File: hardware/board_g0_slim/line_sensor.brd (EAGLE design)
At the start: 100 x 31.3 mm, 62 parts, among them J1 XF2L-0535-1, Q1 BSS123

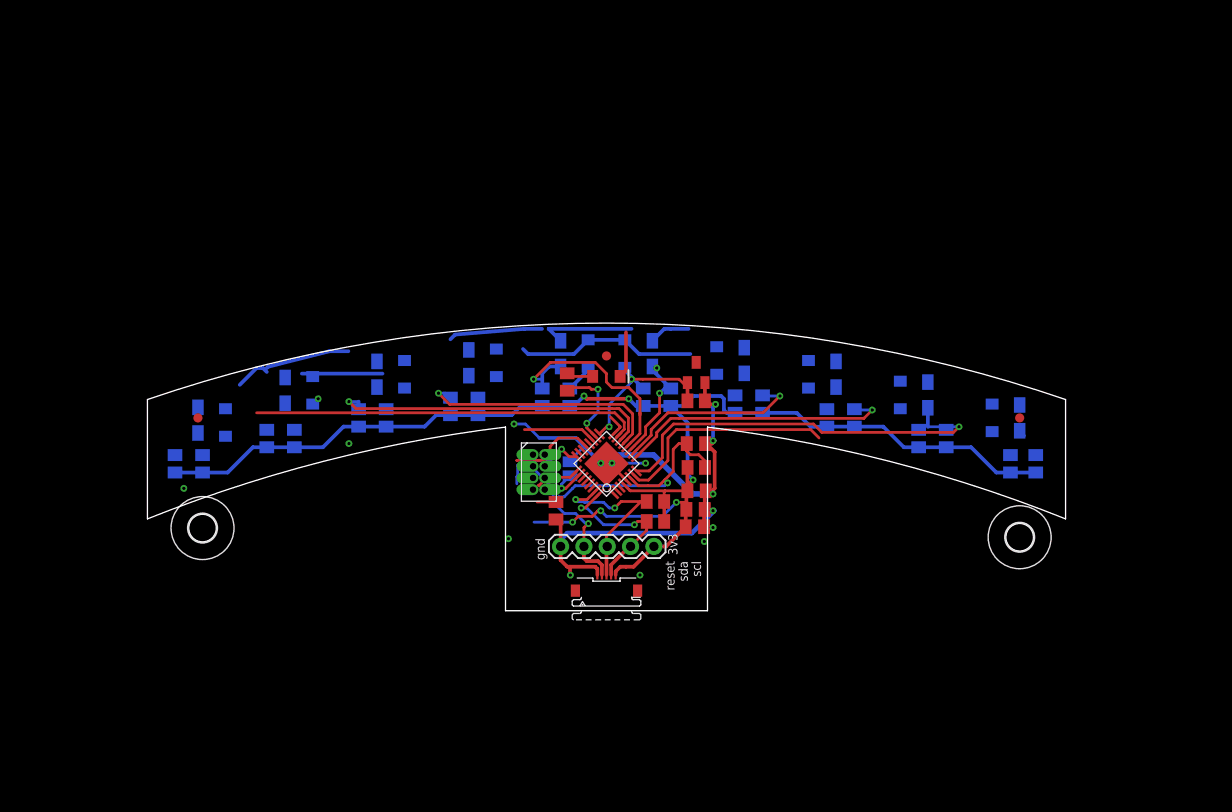
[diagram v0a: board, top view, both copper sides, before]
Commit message: demo codes, cleaned up
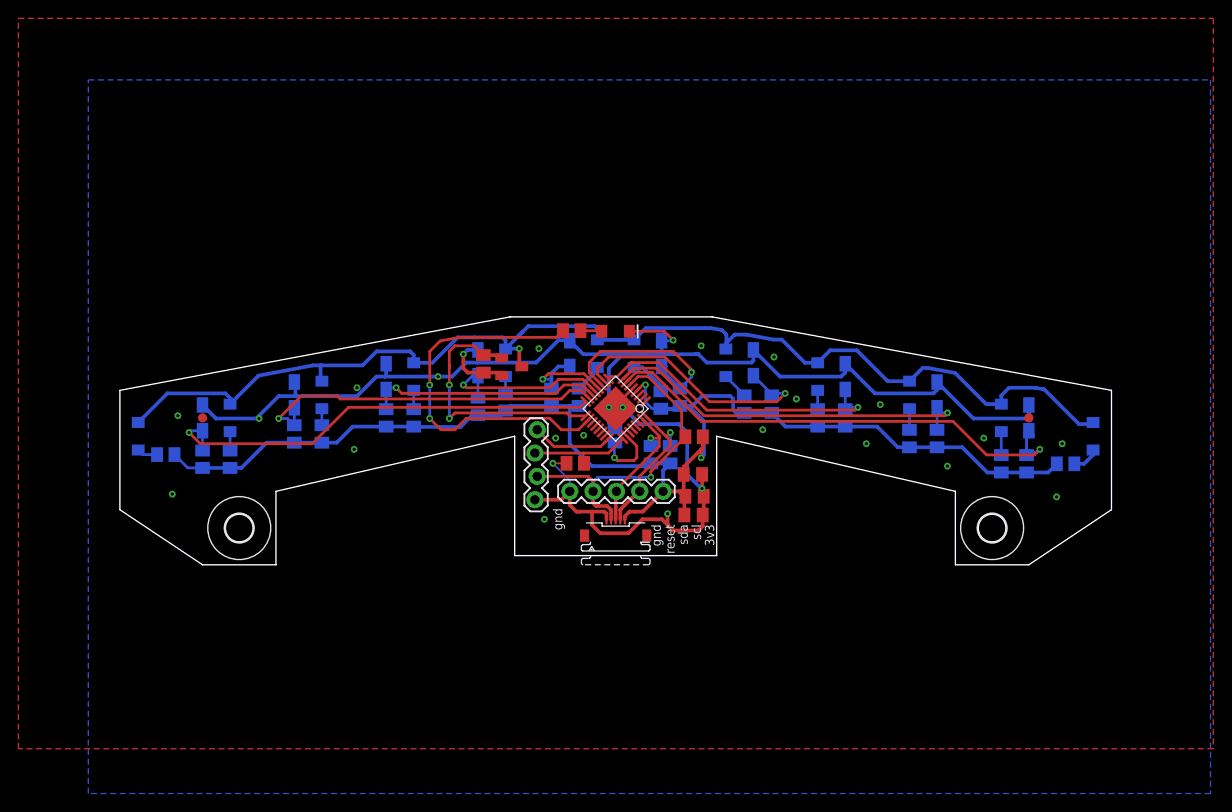
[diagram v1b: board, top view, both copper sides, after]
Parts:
- removed C4: 10n, rcl:C0805K
- removed U$11: FIDUCIAL, borkedlabs-misc:FIDUCIAL_1MM
- removed U$15: DEBUG_CON, my_library:HEADER_4X2_1.27
- added D12, D13: WHITE, SparkFun-LED:LED-1206
- added J3: (no value), SparkFun-Connectors:1X04_LOCK
- added R27, R28: 330, rcl:M0805
- moved R21 23.5 mm to (40.6, 45.9), turned to 90 degrees
- moved Q1 20.1 mm to (43.7, 45.6), turned to 270 degrees
- moved R23 7.44 mm to (60.9, 36.0), flipped to the bottom, turned to 270 degrees
- moved J1 6.08 mm to (55.0, 27.0)
- moved J2 6.08 mm to (50.0, 32.0)
- moved U$14 6.08 mm to (55.0, 41.0), turned to 225 degrees
- moved SJ1 6.06 mm to (54.9, 38.0)
- moved C2 5.70 mm to (63.4, 33.8)
- moved R26 5.61 mm to (50.2, 49.5), turned to 180 degrees
- moved R25 5.57 mm to (50.6, 35.1), turned to 0 degrees
- moved R22 5.12 mm to (58.8, 36.0), flipped to the bottom, turned to 270 degrees
- moved D11 5.02 mm to (55.0, 49.4)
- moved H8 4.00 mm to (14.0, 28.0)
- moved R24 3.34 mm to (63.5, 37.9), turned to 0 degrees
- moved H7 3.16 mm to (96.0, 28.0)
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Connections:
- removed net SWCLK/BOOT: R25.2, U$14.25, U$15.P$6, U$15.P$7
- new net N$13: D12.A, R27.1
- new net N$14: D13.A, R28.1
- new net SWCLK: J3.3, R25.2, U$14.25
- net +3V3: now also R27.2, R28.2; no longer U$15.P$1
- net GND: now also J3.1; no longer C4.2, U$15.P$4
- net N$11: now also D12.C, D13.C
- net RESET: now also J3.2; no longer C4.1, U$15.P$5
- net SWDIO: now also J3.4; no longer U$15.P$8
- net UART_RX: no longer U$15.P$3
- net UART_TX: no longer U$15.P$2
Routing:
- net N$11: track 29.4 -> 132.6 mm, vias 0 -> 1
- net GND: track 136.4 -> 193.5 mm, vias 17 -> 27
- net ADC9: track 2.56 -> 49.3 mm, vias 0 -> 1
- net LED: track 9.71 -> 42.0 mm
- net ADC0: track 25.4 -> 54.6 mm, vias 0 -> 1
- net ADC5: track 25.5 -> 11.9 mm
- net LED_CONTROL: track 17.7 -> 29.4 mm
- net SWCLK: track 0.00 -> 11.4 mm
- net ADC7: track 35.9 -> 25.8 mm
- net ADC4: track 12.2 -> 22.0 mm
- net UART_RX: track 9.60 -> 0.00 mm
- net ADC3: track 20.9 -> 29.9 mm
- net +3V3: track 160.9 -> 152.3 mm, vias 6 -> 2
- net RESET: track 44.5 -> 36.2 mm, vias 2 -> 1
- net UART_TX: track 7.94 -> 0.00 mm
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- added copper zone on layer 1, net GND
- added copper zone on layer 16, net GND
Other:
- board size 100 x 31.3 mm -> 108 x 27 mm
- board text removed: "BOOT"
- board text removed: "UART_RX"
- board text removed: "UART_TX"
